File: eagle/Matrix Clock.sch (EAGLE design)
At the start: 22 parts, among them IC1 LM1117MPX-3.3, IC4 MAX7219CWG, IC5 MAX7219CWG, IC6 MAX7219CWG, IC7 MAX7219CWG

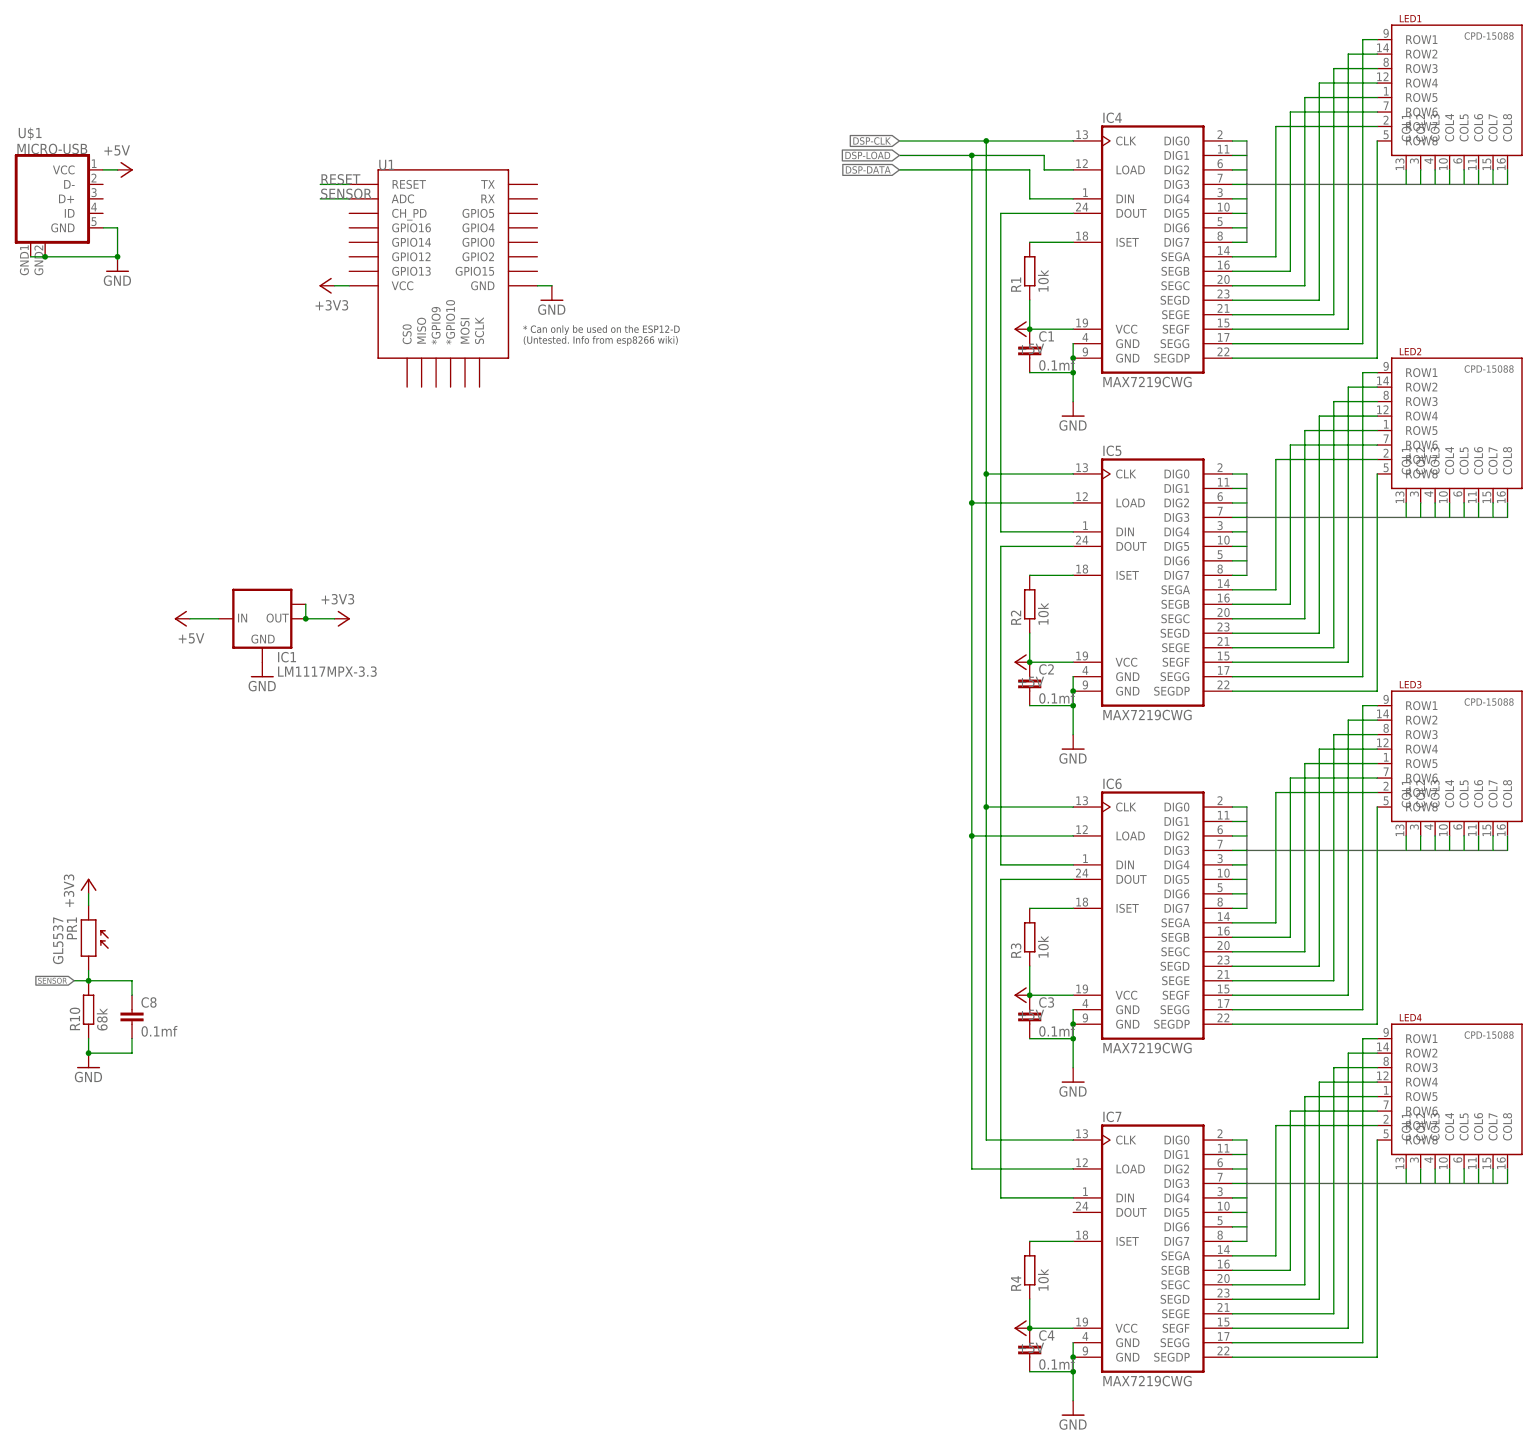
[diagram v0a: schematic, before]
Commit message: .
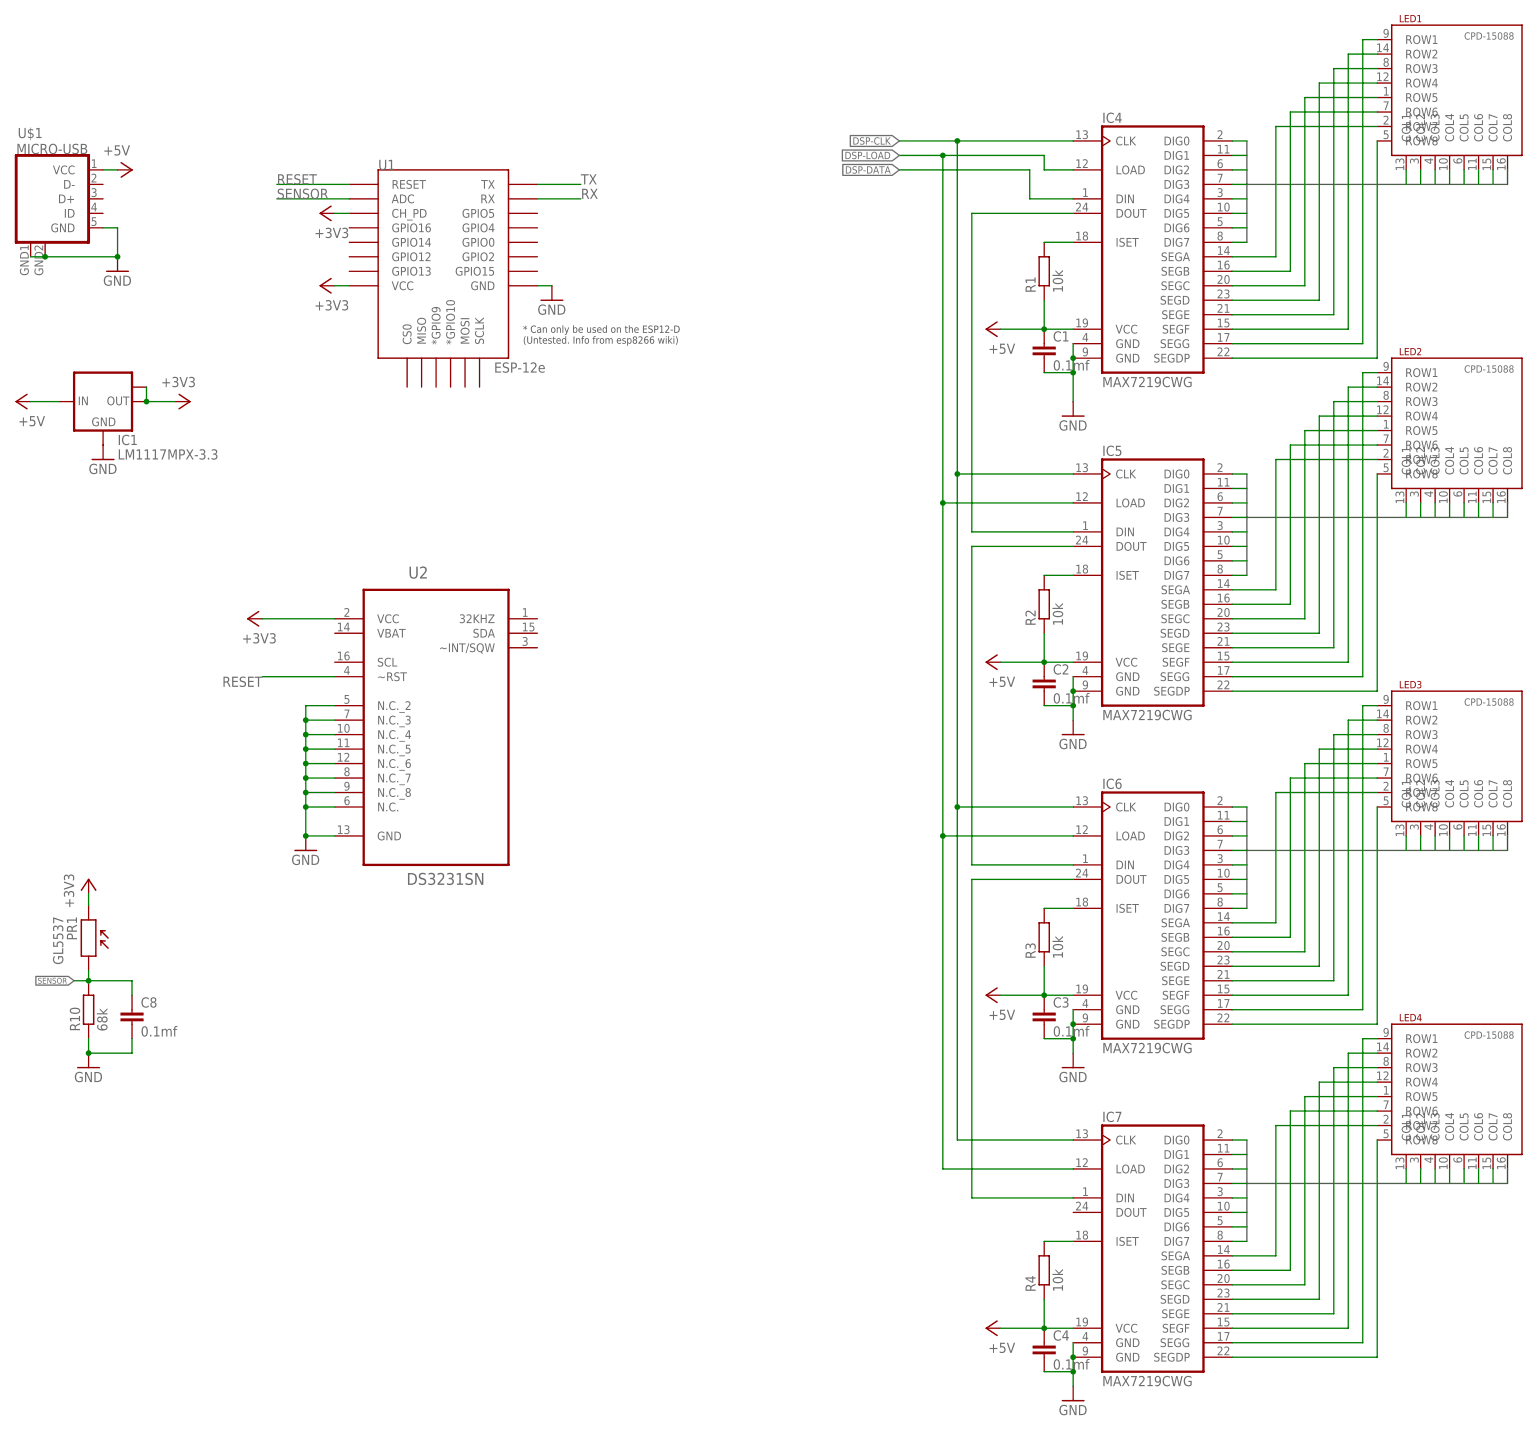
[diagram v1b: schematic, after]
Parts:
- added U2: DS3231SN, DS3231SN:DS3231SN
- U1: value (none) -> ESP-12e
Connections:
- new net RX: U1.RX
- new net TX: U1.TX
- net +3V3: now also U1.CH_PD, U2.VCC
- net GND: now also U2.GND, U2.N.C., U2.N.C._2, U2.N.C._3, U2.N.C._4, U2.N.C._5, U2.N.C._6, U2.N.C._7, U2.N.C._8
- net RESET: now also U2.~RST
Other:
- moved on the sheet: C1, C2, C3, C4, IC1, R1, R2, R3, R4
